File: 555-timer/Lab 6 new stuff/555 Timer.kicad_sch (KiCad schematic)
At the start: 10 parts, among them U1 

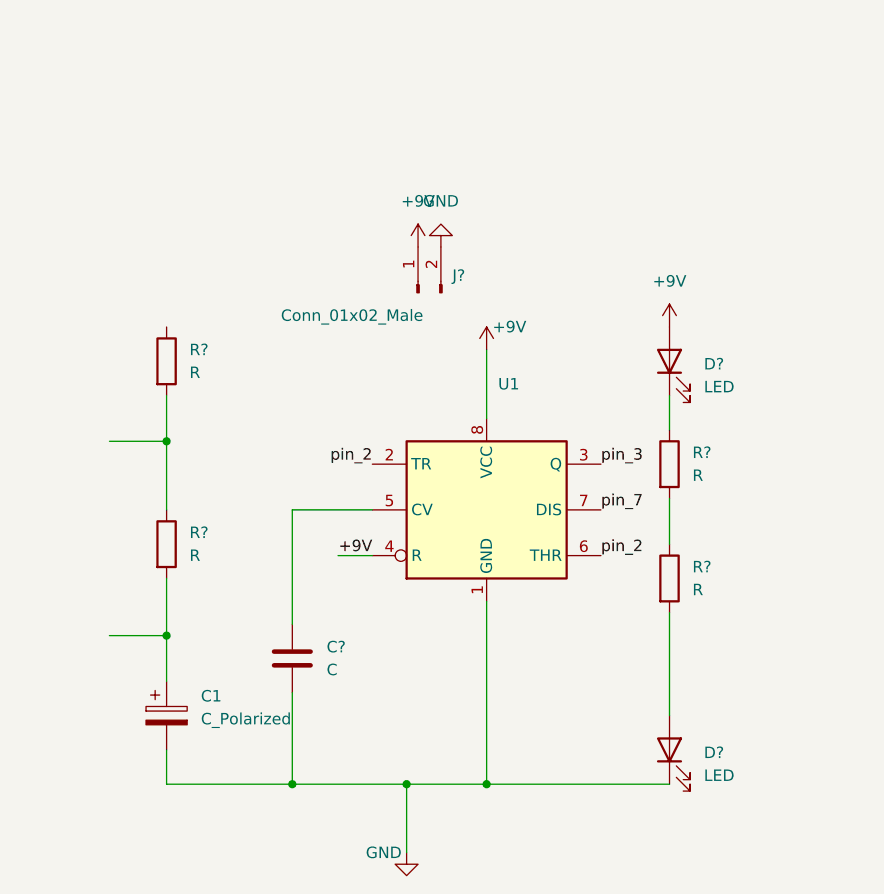
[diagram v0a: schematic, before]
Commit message: lab 6 footprint schematics
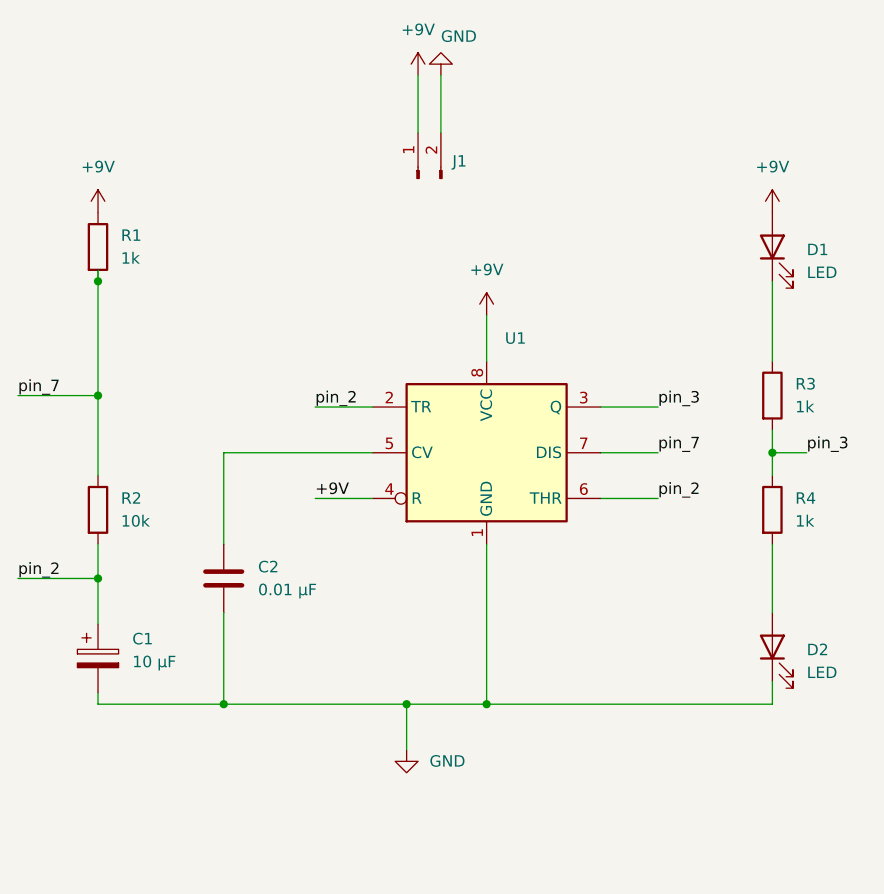
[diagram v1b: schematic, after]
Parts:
- removed C?: C, symbol Device:C
- removed D? (x2): LED, symbol Device:LED
- removed J?: Conn_01x02_Male, symbol Connector:Conn_01x02_Male
- removed R? (x4): R, symbol Device:R
- added C2: 0.01 μF, Capacitor_SMD:C_0805_2012Metric_Pad1.18x1.45mm_HandSolder, symbol Device:C
- added D1, D2: LED, LED_SMD:LED_1206_3216Metric_Pad1.42x1.75mm_HandSolder, symbol Device:LED
- added J1: (no value), TerminalBlock:TerminalBlock_bornier-2_P5.08mm, symbol Connector:Conn_01x02_Male
- added R1, R3, R4: 1k, Resistor_SMD:R_0805_2012Metric_Pad1.20x1.40mm_HandSolder, symbol Device:R
- added R2: 10k, Resistor_SMD:R_0805_2012Metric_Pad1.20x1.40mm_HandSolder, symbol Device:R
- C1: value C_Polarized -> 10 μF; footprint (none) -> Capacitor_Tantalum_SMD:CP_EIA-3216-18_Kemet-A_Pad1.58x1.35mm_HandSolder
- U1: footprint Package_SO:SOIC-8_3.9x4.9mm_P1.27mm -> Package_SO:SOIC-8-1EP_3.9x4.9mm_P1.27mm_EP2.29x3mm
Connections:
- net +9V: now also D1.2 (A), J1.1 (Pin_1), R1.1
- net GND: now also C2.2, D2.1 (K), J1.2 (Pin_2)
- net pin_2: now also C1.1, R2.2
- net pin_3: now also R3.2, R4.1
- net pin_7: now also R1.2, R2.1
- net at U1.5 (CV): now also C2.1
- new net: D2.2 (A), R4.2
- new net: D1.1 (K), R3.1
